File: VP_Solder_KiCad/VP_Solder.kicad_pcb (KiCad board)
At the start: 2 copper layers, 281 x 94.4 mm, 170 parts, among them J1 Conn_01x04, SW1 SW_Push, SW2 SW_Push, U1 STM32F072CBTx, U2 XC6206PxxxMR, U3 USBLC6-2SC6

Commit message: final changes, drc fixes
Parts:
- removed R2, R3: 22, Resistor_SMD:R_0201_0603Metric
- moved U3 3.31 mm to (112.8, 87.8)
- moved C8 2.45 mm to (96.7, 98.4), turned to 180 degrees
- moved C9 0.91 mm to (99.7, 113.9)
- moved COL2 0.89 mm to (127.4, 103.4)
- moved C6 0.84 mm to (97.6, 100.7), turned to 90 degrees
- moved D14 0.36 mm to (341.1, 81.8)
- moved C4 0.31 mm to (98.9, 113.7)
- moved J1 0.18 mm to (119.0, 87.8)
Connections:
- U1 pad 32: /RES_D- -> /ESD_D-
- U1 pad 33: /RES_D+ -> /ESD_D+
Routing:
- net /ESD_D-: track 3.28 -> 24.8 mm
- net /ESD_D+: track 3.15 -> 23.3 mm
- net /RES_D-: track 17.5 -> 0.00 mm
- net /RES_D+: track 16.4 -> 0.00 mm
- net /USB_D+: track 6.40 -> 3.20 mm
- net /USB_D-: track 6.27 -> 3.22 mm
- net +3.3V: track 67.2 -> 65.2 mm
- net /NRST: track 34.1 -> 32.4 mm
- net +5V: track 36.4 -> 35.4 mm
- net /COL2: track 115.6 -> 114.7 mm
- net GND: track 21.0 -> 21.6 mm, vias 18 -> 19
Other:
- board text added: "BOOT"
- board text added: "RESET"

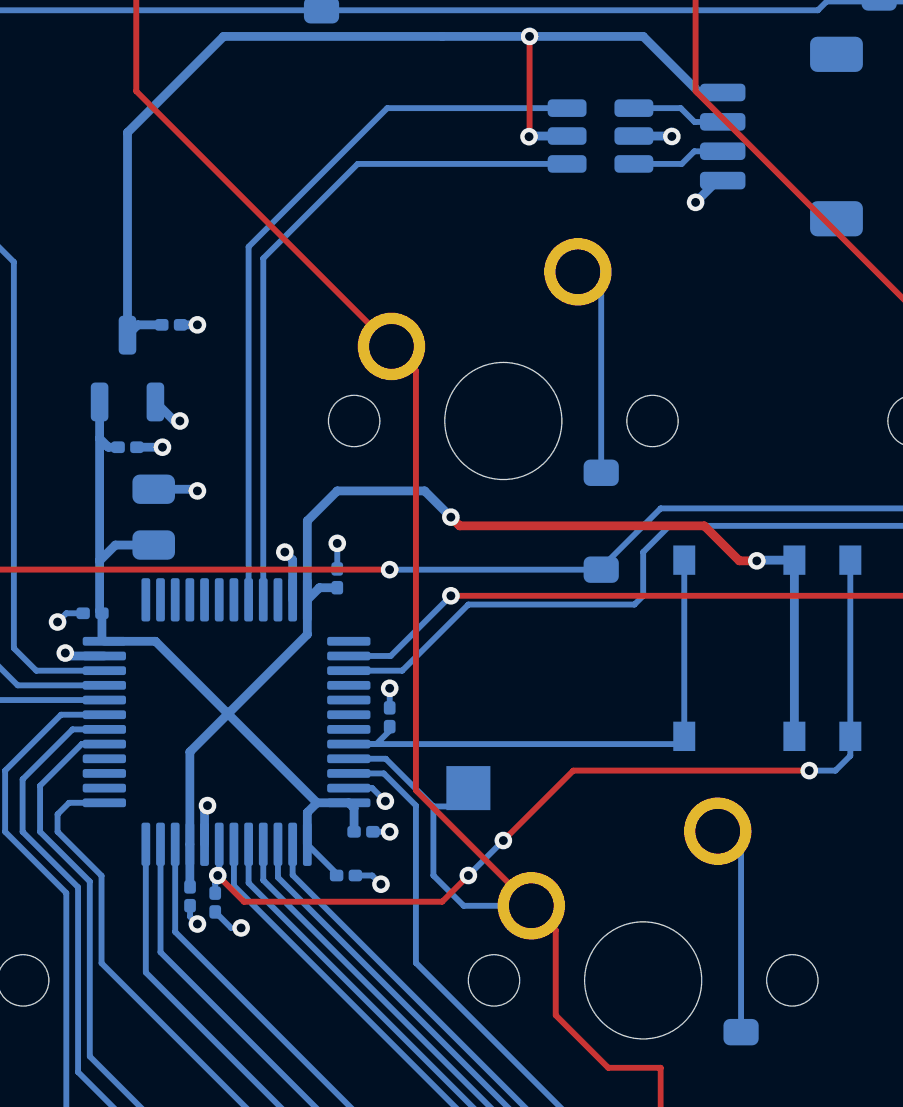
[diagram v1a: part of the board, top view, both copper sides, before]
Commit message: Cleaup
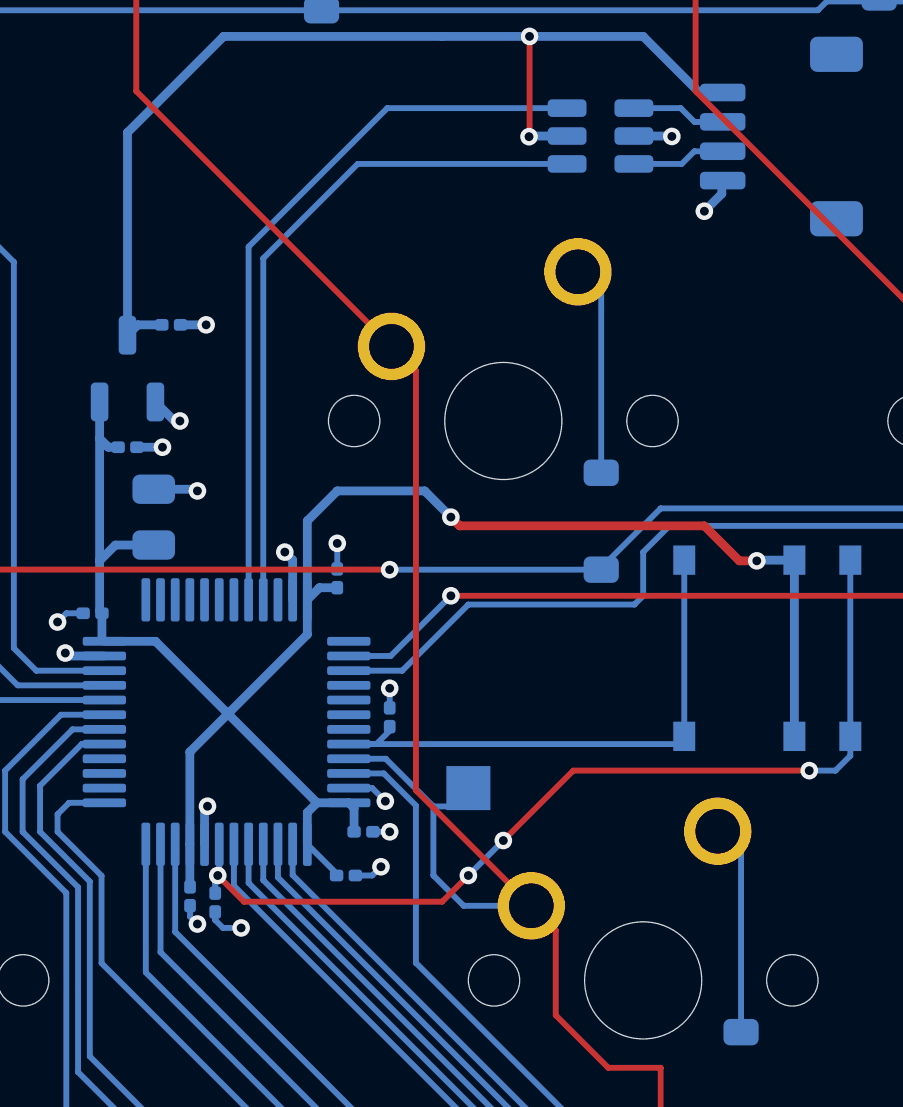
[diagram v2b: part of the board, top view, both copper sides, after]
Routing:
- net GND: track 21.6 -> 22.1 mm
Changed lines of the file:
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@@
 	)
 	(via
-		(at 105.370292 113.24838)
+		(at 105.370292 112.653068)
 		(size 0.6)
 		(drill 0.3)
@@
 	)
 	(via
-		(at 116.085908 90.027217)
+		(at 116.383564 90.328868)
 		(size 0.6)
 		(drill 0.3)
@@
 	)
 	(via
-		(at 99.46266 110.569476)
+		(at 99.46266 110.59222)
 		(size 0.6)
 		(drill 0.3)
@@
 	)
 	(via
-		(at 99.119516 94.198396)
+		(at 99.417172 94.198396)
 		(size 0.6)
 		(drill 0.3)
@@
 	)
 	(segment
+		(start 116.978876 89.314867)
+		(end 117.008189 89.285554)
+		(width 0.3)
+		(layer "B.Cu")
+		(net "GND")
+	)
+	(segment
 		(start 97.058268 98.36558)
 		(end 97.928892 98.36558)
@@
 	)
 	(segment
-		(start 100.270507 114.73666)
+		(start 105.370292 112.653068)
+		(end 105.072636 112.950724)
+		(width 0.2)
+		(layer "B.Cu")
+		(net "GND")
+	)
+	(segment
+		(start 116.978876 89.733556)
+		(end 116.978876 89.314867)
+		(width 0.3)
+		(layer "B.Cu")
+		(net "GND")
+	)
+	(segment
+		(start 97.631236 99.796828)
+		(end 99.062484 99.796828)
+		(width 0.3)
+		(layer "B.Cu")
+		(net "GND")
+	)
+	(segment
+		(start 113.983978 87.76816)
+		(end 115.262764 87.76816)
+		(width 0.3)
+		(layer "B.Cu")
+		(net "GND")
+	)
+	(segment
+		(start 105.073595 109.975123)
+		(end 104.27516 109.975123)
+		(width 0.2)
+		(layer "B.Cu")
+		(net "GND")
+	)
+	(segment
+		(start 105.51912 110.420648)
+		(end 105.073595 109.975123)
+		(width 0.2)
+		(layer "B.Cu")
+		(net "GND")
+	)
+	(segment
+		(start 94.720475 105.475123)
+		(end 95.95016 105.475123)
+		(width 0.3)
+		(layer "B.Cu")
+		(net "GND")
+	)
+	(segment
+		(start 98.546548 94.198396)
+		(end 99.417172 94.198396)
+		(width 0.3)
+		(layer "B.Cu")
+		(net "GND")
+	)
+	(segment
+		(start 123.527308 102.235108)
+		(end 125.081212 102.235108)
+		(width 0.2)
+		(layer "B.Cu")
+		(net "GND")
+	)
+	(segment
+		(start 103.882012 102.51042)
+		(end 103.882012 101.639796)
+		(width 0.2)
+		(layer "B.Cu")
+		(net "GND")
+	)
+	(segment
+		(start 98.868533 114.352316)
+		(end 98.868533 113.978492)
+		(width 0.2)
+		(layer "B.Cu")
+		(net "GND")
+	)
+	(segment
+		(start 99.119516 114.603299)
+		(end 98.868533 114.352316)
+		(width 0.2)
+		(layer "B.Cu")
+		(net "GND")
+	)
+	(segment
+		(start 99.725211 114.469204)
 		(end 99.725211 114.191364)
 		(width 0.2)
-		(layer "B.Cu")
-		(net "GND")
-	)
-	(segment
-		(start 99.36266 111.887623)
-		(end 99.36266 110.669476)
-		(width 0.3)
 		(layer "B.Cu")
 		(net "GND")
@@
 	)
 	(segment
-		(start 97.631236 99.796828)
-		(end 99.062484 99.796828)
-		(width 0.3)
-		(layer "B.Cu")
-		(net "GND")
-	)
-	(segment
-		(start 113.983978 87.76816)
-		(end 115.262764 87.76816)
-		(width 0.3)
-		(layer "B.Cu")
-		(net "GND")
-	)
-	(segment
-		(start 105.073595 109.975123)
-		(end 104.27516 109.975123)
-		(width 0.2)
-		(layer "B.Cu")
-		(net "GND")
-	)
-	(segment
-		(start 105.51912 110.420648)
-		(end 105.073595 109.975123)
-		(width 0.2)
-		(layer "B.Cu")
-		(net "GND")
-	)
-	(segment
-		(start 94.720475 105.475123)
-		(end 95.95016 105.475123)
-		(width 0.3)
-		(layer "B.Cu")
-		(net "GND")
-	)
-	(segment
-		(start 123.527308 102.235108)
-		(end 125.081212 102.235108)
-		(width 0.2)
-		(layer "B.Cu")
-		(net "GND")
-	)
-	(segment
-		(start 100.607796 114.73666)
-		(end 100.270507 114.73666)
-		(width 0.2)
-		(layer "B.Cu")
-		(net "GND")
-	)
-	(segment
-		(start 103.882012 102.51042)
-		(end 103.882012 101.639796)
-		(width 0.2)
-		(layer "B.Cu")
-		(net "GND")
-	)
-	(segment
-		(start 98.868533 114.352316)
-		(end 98.868533 113.978492)
-		(width 0.2)
-		(layer "B.Cu")
-		(net "GND")
-	)
-	(segment
-		(start 99.119516 114.603299)
-		(end 98.868533 114.352316)
-		(width 0.2)
-		(layer "B.Cu")
-		(net "GND")
-	)
-	(segment
-		(start 105.370292 113.24838)
-		(end 105.072636 112.950724)
-		(width 0.2)
+		(start 116.383564 90.328868)
+		(end 116.978876 89.733556)
+		(width 0.3)
 		(layer "B.Cu")
 		(net "GND")
@@
 	)
 	(segment
+		(start 99.36266 110.669476)
+		(end 99.36266 111.887623)
+		(width 0.3)
+		(layer "B.Cu")
+		(net "GND")
+	)
+	(segment
 		(start 94.654676 104.021044)
 		(end 94.35702 104.3187)
@@
 	)
 	(segment
-		(start 98.546548 94.198396)
-		(end 99.119516 94.198396)
-		(width 0.3)
-		(layer "B.Cu")
-		(net "GND")
-	)
-	(segment
-		(start 116.085908 90.027217)
-		(end 116.827571 89.285554)
-		(width 0.3)
-		(layer "B.Cu")
-		(net "GND")
-	)
-	(segment
-		(start 99.36266 110.669476)
-		(end 99.46266 110.569476)
+		(start 99.992667 114.73666)
+		(end 99.725211 114.469204)
+		(width 0.2)
+		(layer "B.Cu")
+		(net "GND")
+	)
+	(segment
+		(start 99.439916 110.59222)
+		(end 99.36266 110.669476)
 		(width 0.3)
 		(layer "B.Cu")
@@
 	)
 	(segment
+		(start 99.46266 110.59222)
+		(end 99.439916 110.59222)
+		(width 0.3)
+		(layer "B.Cu")
+		(net "GND")
+	)
+	(segment
 		(start 102.096076 101.937452)
 		(end 102.36266 102.204036)
@@
 	)
 	(segment
-		(start 116.827571 89.285554)
-		(end 117.008189 89.285554)
-		(width 0.3)
-		(layer "B.Cu")
-		(net "GND")
+		(start 100.607796 114.73666)
+		(end 99.992667 114.73666)
+		(width 0.2)
+		(layer "B.Cu")
+		(net "GND")
